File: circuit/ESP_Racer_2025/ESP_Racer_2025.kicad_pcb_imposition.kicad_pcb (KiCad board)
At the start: 2 copper layers, 20 x 35 mm, 19 parts, among them IC1 XCL102D333CR-G, J1 Conn_LED_1, J2 Conn_LED_2, J3 Conn_Servo, U1 DRV8835DSST, U2 SFV12R-2STE1LF, U3 ESP32-C3-WROOM-02

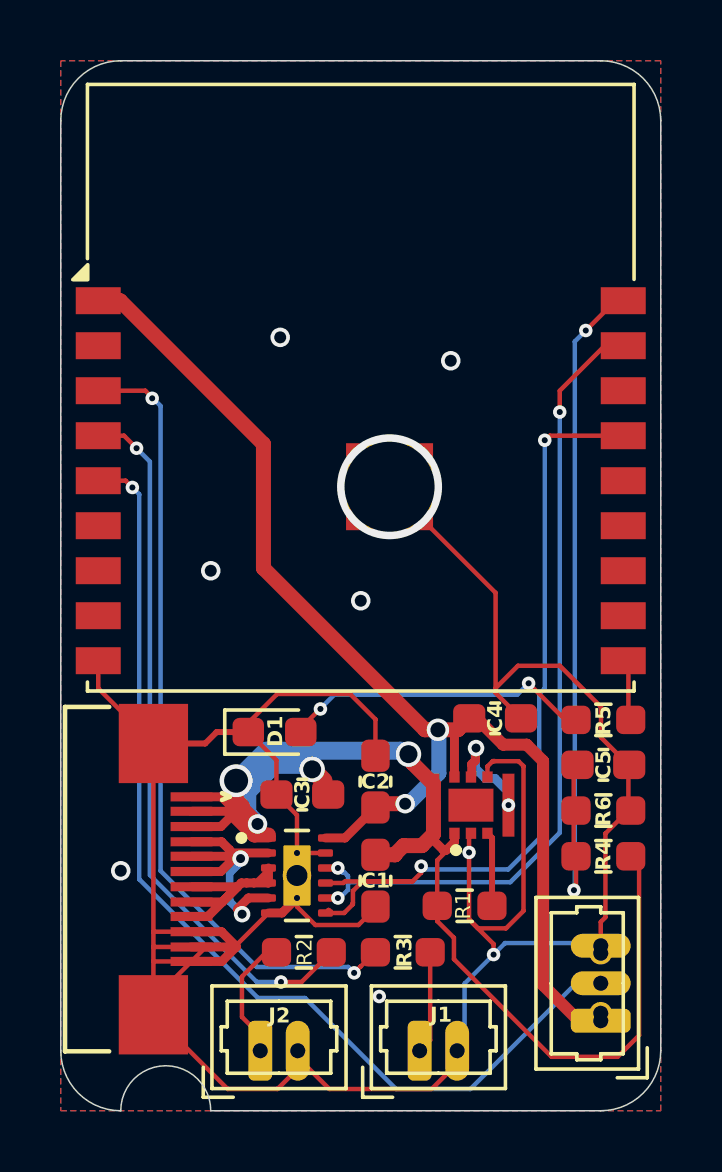
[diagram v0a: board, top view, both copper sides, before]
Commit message: update pcb
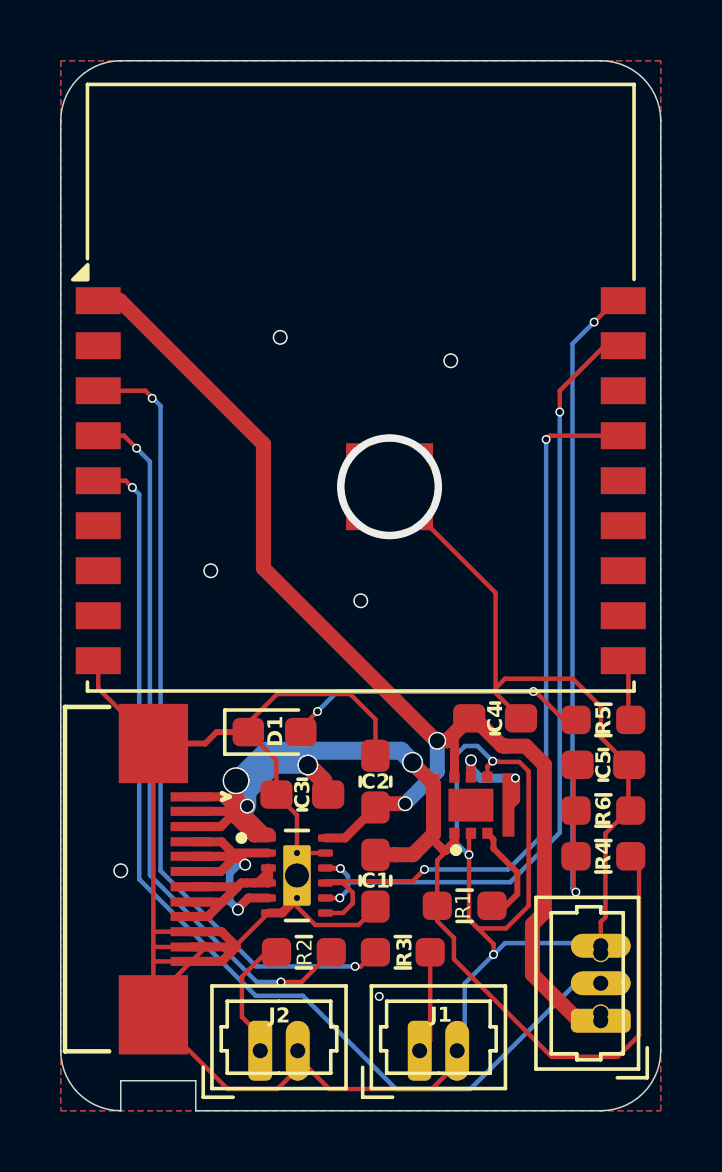
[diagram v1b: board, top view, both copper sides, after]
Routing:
- net GND: track 102.6 -> 107.4 mm, vias 9 -> 10
- net AIN 2: track 27.5 -> 26.2 mm
- net +BATT: track 46.1 -> 45.0 mm
- net Net-(IC1-CE): track 2.48 -> 3.45 mm
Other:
- outline, holes or cut-outs redrawn
